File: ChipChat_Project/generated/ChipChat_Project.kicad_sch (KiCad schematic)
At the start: 0 parts

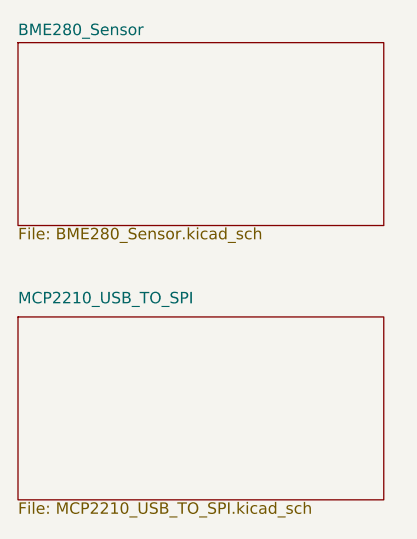
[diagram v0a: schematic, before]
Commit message: 💾 snapshot 2026-02-19_17-31-37
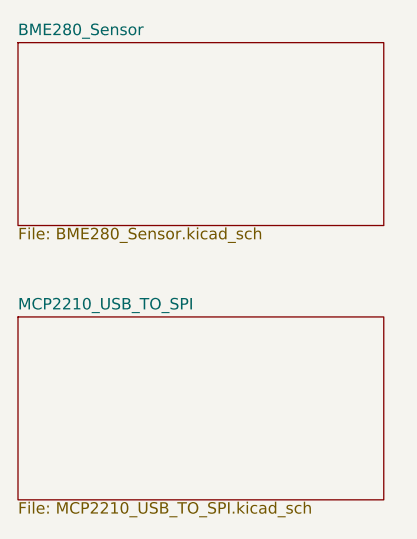
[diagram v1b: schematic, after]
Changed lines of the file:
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@@
 		)
 		(property "Sheetfile" "BME280_Sensor.kicad_sch"
-			(at 30.48 51 0)
+			(at 30.48 51.0 0)
 			(effects
 				(font
@@
 		)
 		(property "Sheetname" "MCP2210_USB_TO_SPI"
-			(at 30.48 59.6 0)
+			(at 30.48 60.28 0)
 			(effects
 				(font
@@
 		)
 		(property "Sheetfile" "MCP2210_USB_TO_SPI.kicad_sch"
-			(at 30.48 81.5 0)
+			(at 30.48 81.48 0)
 			(effects
 				(font
